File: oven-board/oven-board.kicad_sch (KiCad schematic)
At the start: 40 parts, among them J1 Temp Sensor Conn, J2 heating element 1, J3 wall outlet, J4 12V Power Supply, J5 heating element 2, J6 wall outlet, J7 switch1, J8 switch1, K1 G2RL-1A-E, K2 G2RL-1A-E, SW1 SW_Push, SW2 SW_Push, SW3 SW_Push, SW4 SW_Push, SW5 SW_Push, SW6 SW_Push, U1 SZNUD3124LT1G, U2 L78L09_TO92, U3 NUCLEO-L432KC, U4 SZNUD3124LT1G, U5 NHD-C0220BIZ, U6 INA826AIDR, U7 MCP1792x-3302xDB

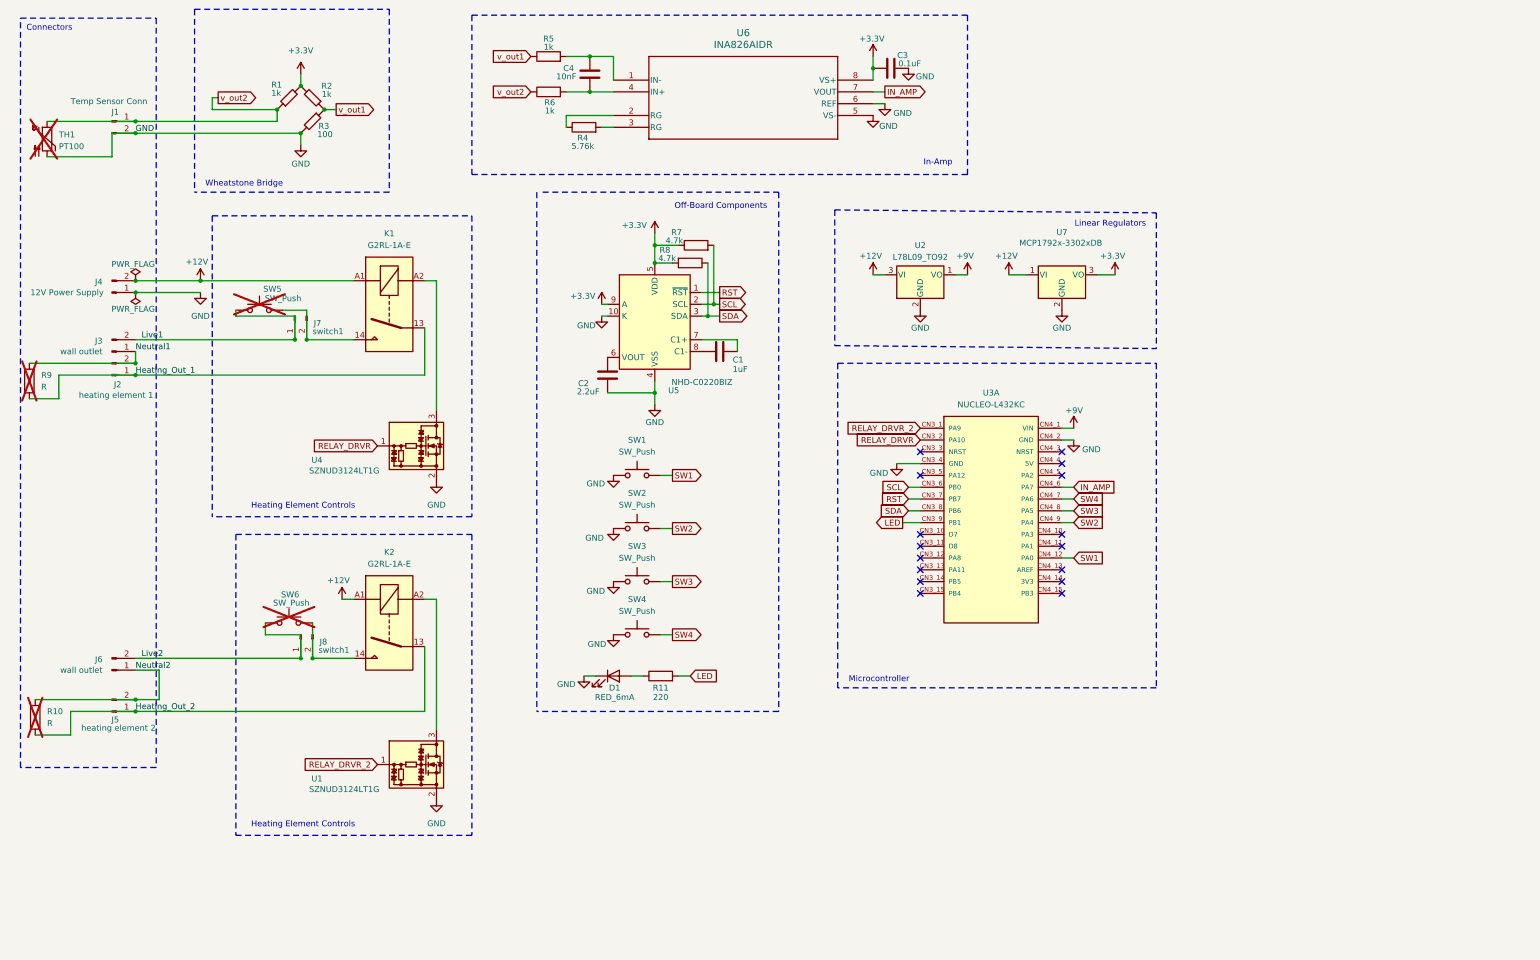
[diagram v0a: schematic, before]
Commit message: Imported board settings from VCU
Still need to actually change the sizes of traces
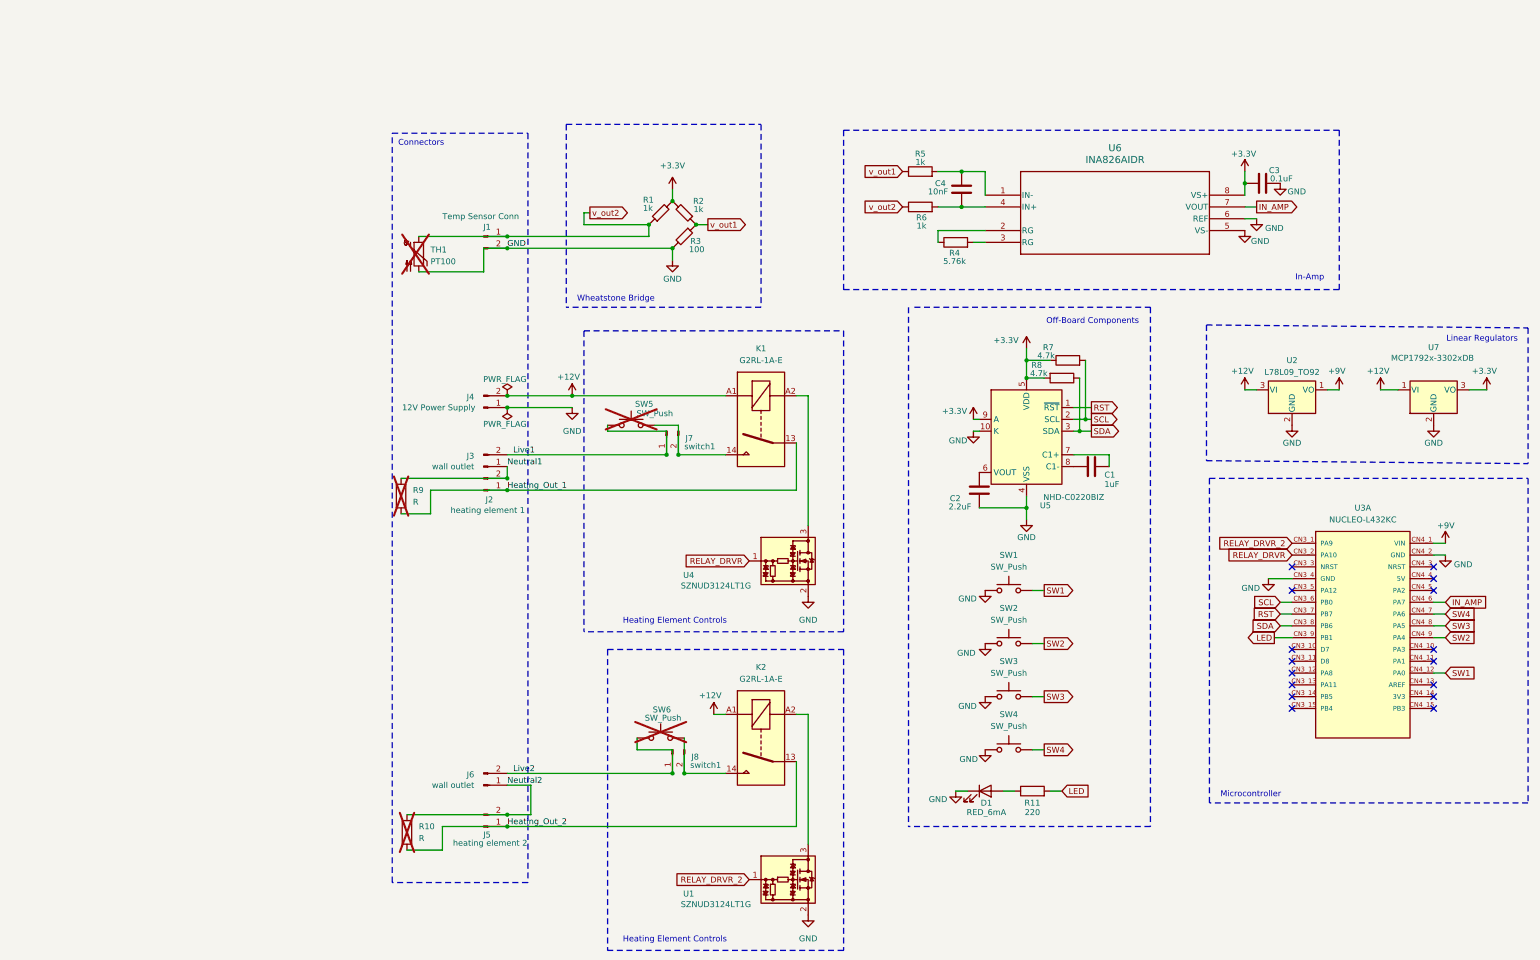
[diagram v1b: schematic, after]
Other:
- moved on the sheet: C1, C2, C3, C4, D1, J1, J2, J3, J4, J5, J6, J7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
